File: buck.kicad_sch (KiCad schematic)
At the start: 0 parts

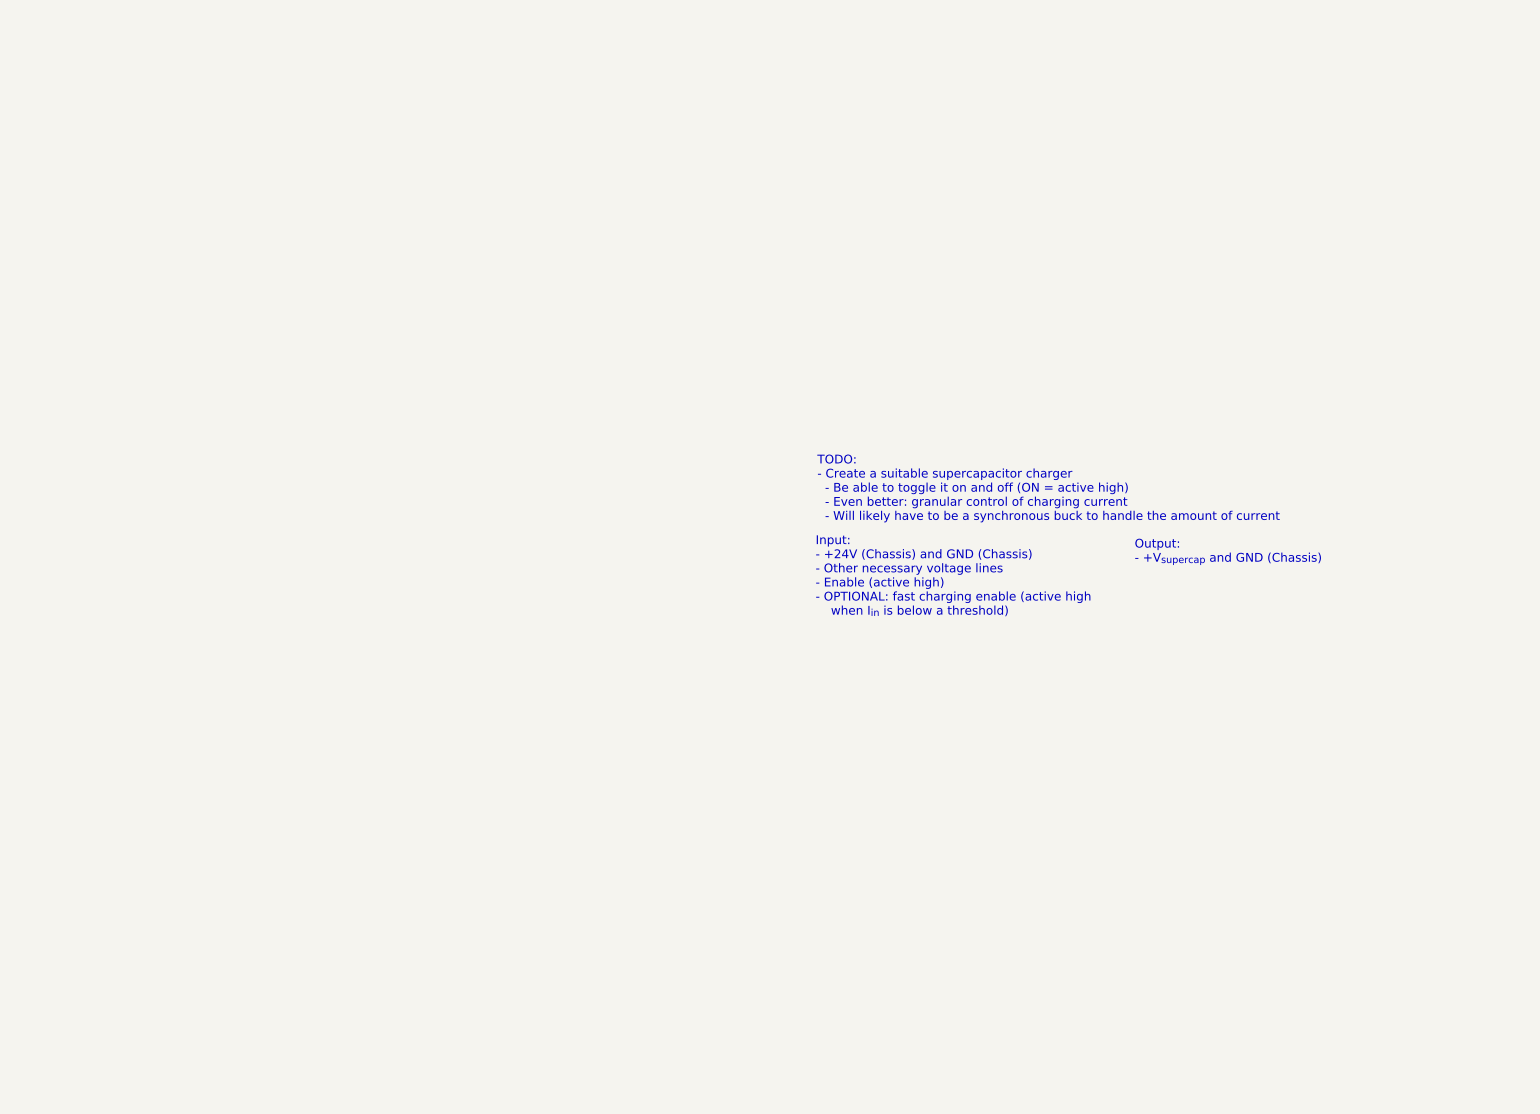
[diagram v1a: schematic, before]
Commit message: Finishing buck charger
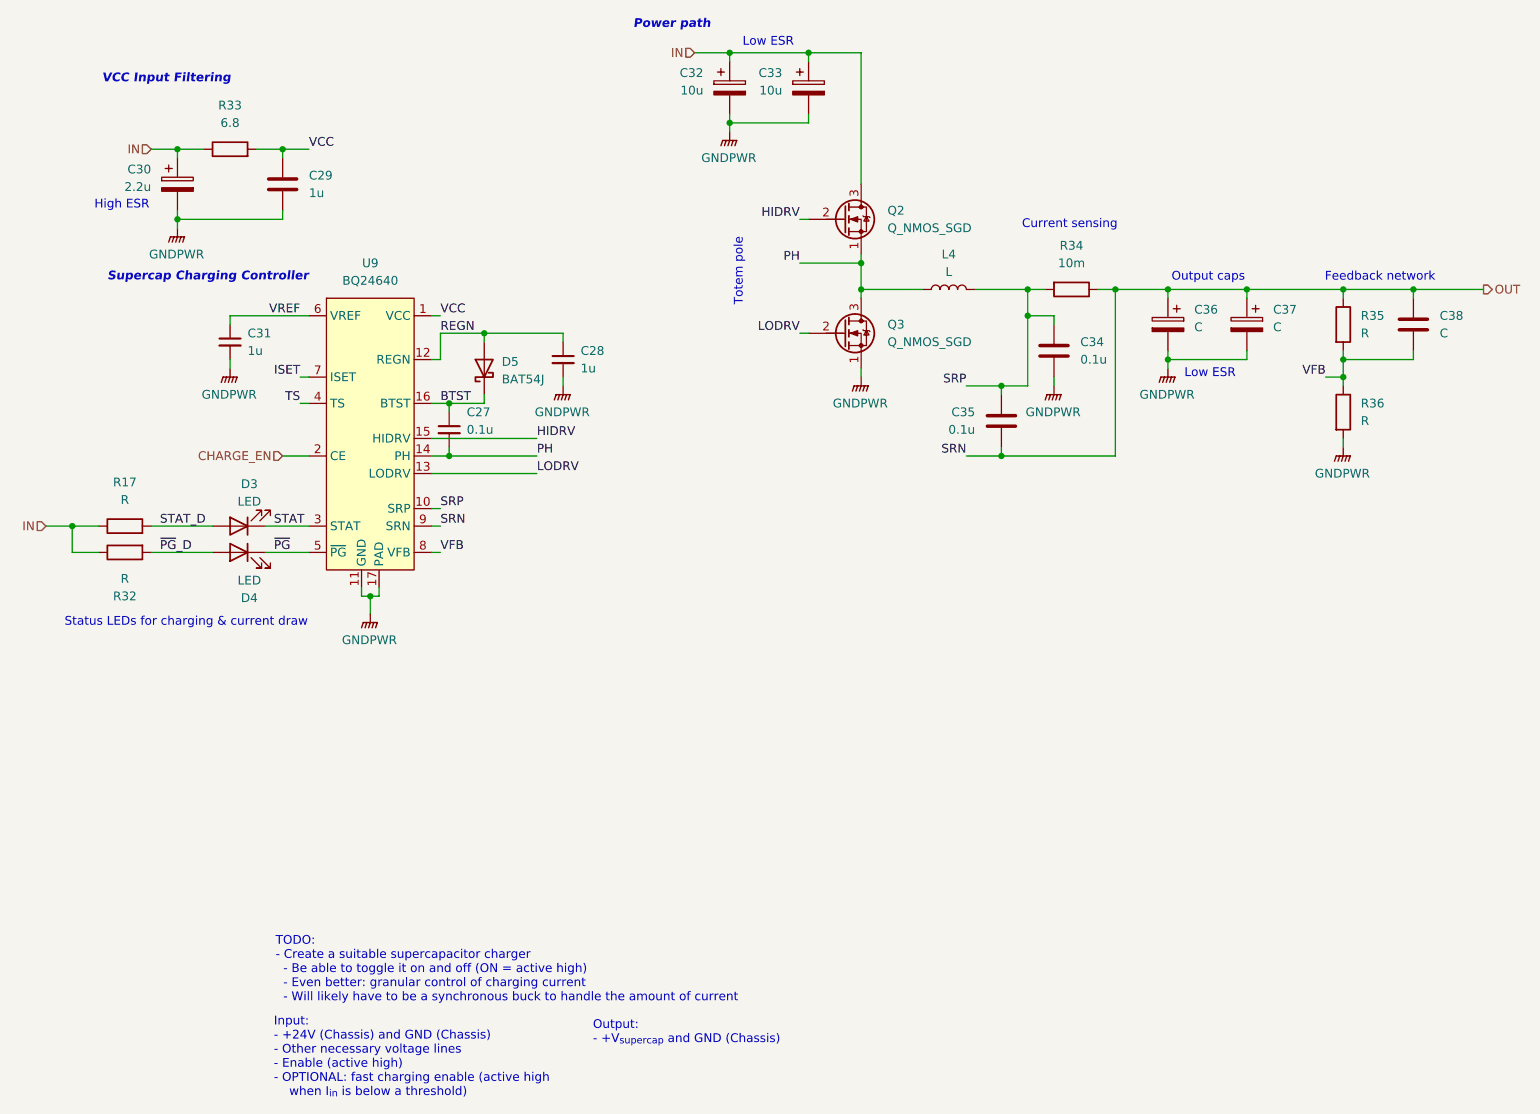
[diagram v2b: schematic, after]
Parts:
- added C27: 0.1u, Capacitor_SMD:C_0603_1608Metric_Pad1.08x0.95mm_HandSolder, symbol Device:C_Small
- added C28, C31: 1u, Capacitor_SMD:C_0603_1608Metric_Pad1.08x0.95mm_HandSolder, symbol Device:C_Small
- added C29: 1u, Capacitor_SMD:C_0603_1608Metric_Pad1.08x0.95mm_HandSolder, symbol Device:C
- added C30: 2.2u, symbol Device:C_Polarized
- added C32, C33: 10u, symbol Device:C_Polarized
- added C34, C35: 0.1u, Capacitor_SMD:C_0603_1608Metric_Pad1.08x0.95mm_HandSolder, symbol Device:C
- added C36, C37: C, symbol Device:C_Polarized
- added C38: C, Capacitor_SMD:C_0603_1608Metric_Pad1.08x0.95mm_HandSolder, symbol Device:C
- added D3, D4: LED, LED_SMD:LED_0603_1608Metric_Pad1.05x0.95mm_HandSolder, symbol Device:LED
- added D5: BAT54J, Diode_SMD:D_SOD-323F, symbol Diode:BAT54J
- added L4: L, symbol Device:L
- added Q2, Q3: Q_NMOS_SGD, symbol Device:Q_NMOS_SGD
- added R17, R32, R35, R36: R, Resistor_SMD:R_0603_1608Metric_Pad0.98x0.95mm_HandSolder, symbol Device:R
- added R33: 6.8, Resistor_SMD:R_0603_1608Metric_Pad0.98x0.95mm_HandSolder, symbol Device:R
- added R34: 10m, Resistor_SMD:R_0603_1608Metric_Pad0.98x0.95mm_HandSolder, symbol Device:R
- added U9: BQ24640, ! Robomaster ICs:QFN50P350X350X100-17N-D, symbol ! Robomaster ICs:BQ24640
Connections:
- new net BTST: C27.1, D5.1 (K), U9.16 (BTST)
- new net CHARGE_EN: U9.2 (CE)
- new net GNDPWR: C28.2, C29.2, C30.2, C31.2, C32.2, C33.2, C34.2, C36.2, C37.2, Q3.1 (S), R36.2, U9.11 (GND), U9.17 (PAD)
- new net HIDRV: Q2.2 (G), U9.15 (HIDRV)
- new net IN: C30.1, C32.1, C33.1, Q2.3 (D), R17.1, R32.1, R33.1
- new net ISET: U9.7 (ISET)
- new net LODRV: Q3.2 (G), U9.13 (LODRV)
- new net OUT: C35.2, C36.1, C37.1, C38.1, R34.1, R35.1, U9.9 (SRN)
- new net PH: C27.2, L4.1, Q2.1 (S), Q3.3 (D), U9.14 (PH)
- new net REGN: C28.1, D5.2 (A), U9.12 (REGN)
- new net SRP: C34.1, C35.1, L4.2, R34.2, U9.10 (SRP)
- new net STAT: D3.1 (K), U9.3 (STAT)
- new net STAT_D: D3.2 (A), R17.2
- new net TS: U9.4 (TS)
- new net VCC: C29.1, R33.2, U9.1 (VCC)
- new net VFB: C38.2, R35.2, R36.1, U9.8 (VFB)
- new net VREF: C31.1, U9.6 (VREF)
- new net ~{PG}: D4.1 (K), U9.5 (~{PG})
- new net ~{PG}_D: D4.2 (A), R32.2
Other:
- note added: "Current sensing"
- note added: "Feedback network"
- note added: "High ESR"
- note added: "Low ESR"
- note added: "Output caps"
- note added: "Power path"
- note added: "Status LEDs for charging & current draw"
- note added: "Supercap Charging Controller"
- note added: "Totem pole"
- note added: "VCC Input Filtering"
